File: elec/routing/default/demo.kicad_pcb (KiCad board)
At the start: 4 copper layers, 25 x 25 mm, 34 parts, among them U1 ?, U2 ?, U3 ?, U4 ?, U5 ?, U6 KMR211NGLFS (Tactile Switches), U7 ?, U8 ?

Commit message: [DEMO] tweaks
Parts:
- C1, C15, C19, C2: value 25V 1uF X5R Â±10% 0402 Multilayer Ceramic Capacitors MLCC - SMD/SMT ROHS -> 25V 1uF X5R ±10% 0402 Multilayer Ceramic Capacitors MLCC - SMD/SMT ROHS
- C10, C11, C12, C13, C14, C16, C17, C18, C4, C6, C7: value 16V 100nF X7R Â±10% 0402 Multilayer Ceramic Capacitors MLCC - SMD/SMT ROHS -> 16V 100nF X7R ±10% 0402 Multilayer Ceramic Capacitors MLCC - SMD/SMT ROHS
- C3: value 6.3V 10uF X5R Â±20% 0402 Multilayer Ceramic Capacitors MLCC - SMD/SMT ROHS -> 6.3V 10uF X5R ±20% 0402 Multilayer Ceramic Capacitors MLCC - SMD/SMT ROHS
- C5: value 10V 4.7uF X5R Â±20% 0402 Multilayer Ceramic Capacitors MLCC - SMD/SMT ROHS -> 10V 4.7uF X5R ±20% 0402 Multilayer Ceramic Capacitors MLCC - SMD/SMT ROHS
- C8, C9: value 50V 20pF C0G Â±5% 0402 Multilayer Ceramic Capacitors MLCC - SMD/SMT ROHS -> 50V 20pF C0G ±5% 0402 Multilayer Ceramic Capacitors MLCC - SMD/SMT ROHS
- R1, R2: value 62.5mW Thick Film Resistors 50V Â±100ppm/â Â±1% 5.1kÎ© 0402 Chip Resistor - Surface Mount ROHS -> 62.5mW Thick Film Resistors 50V ±100ppm/℃ ±1% 5.1kΩ 0402 Chip Resistor - Surface Mount ROHS
- R3, R4: value 62.5mW Thick Film Resistors 50V Â±100ppm/â Â±1% 10kÎ© 0402 Chip Resistor - Surface Mount ROHS -> 62.5mW Thick Film Resistors 50V ±100ppm/℃ ±1% 10kΩ 0402 Chip Resistor - Surface Mount ROHS
- R5: value 62.5mW Thick Film Resistors 50V Â±100ppm/â Â±1% 1kÎ© 0402 Chip Resistor - Surface Mount ROHS -> 62.5mW Thick Film Resistors 50V ±100ppm/℃ ±1% 1kΩ 0402 Chip Resistor - Surface Mount ROHS
- R6, R7: value 62.5mW Thick Film Resistors 50V Â±100ppm/â Â±1% 27Î© 0402 Chip Resistor - Surface Mount ROHS -> 62.5mW Thick Film Resistors 50V ±100ppm/℃ ±1% 27Ω 0402 Chip Resistor - Surface Mount ROHS

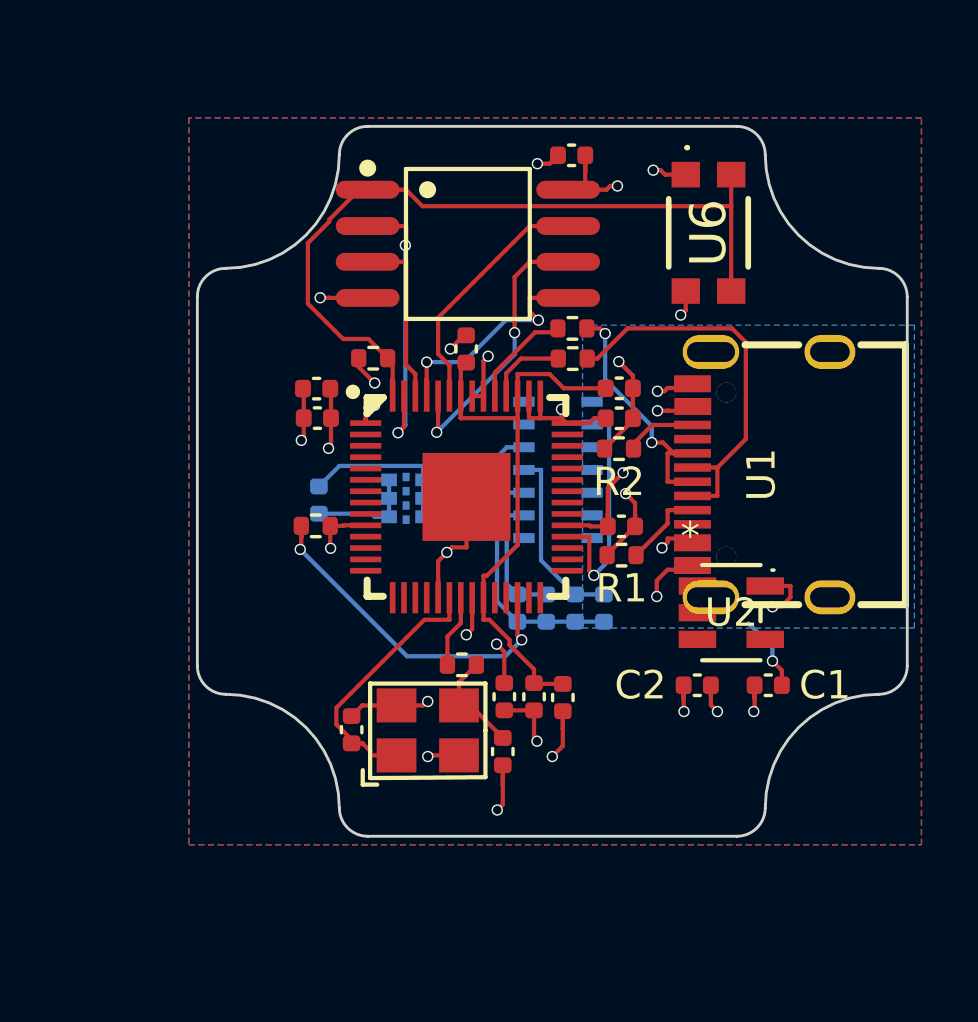
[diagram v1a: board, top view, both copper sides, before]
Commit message: [DEMO] better
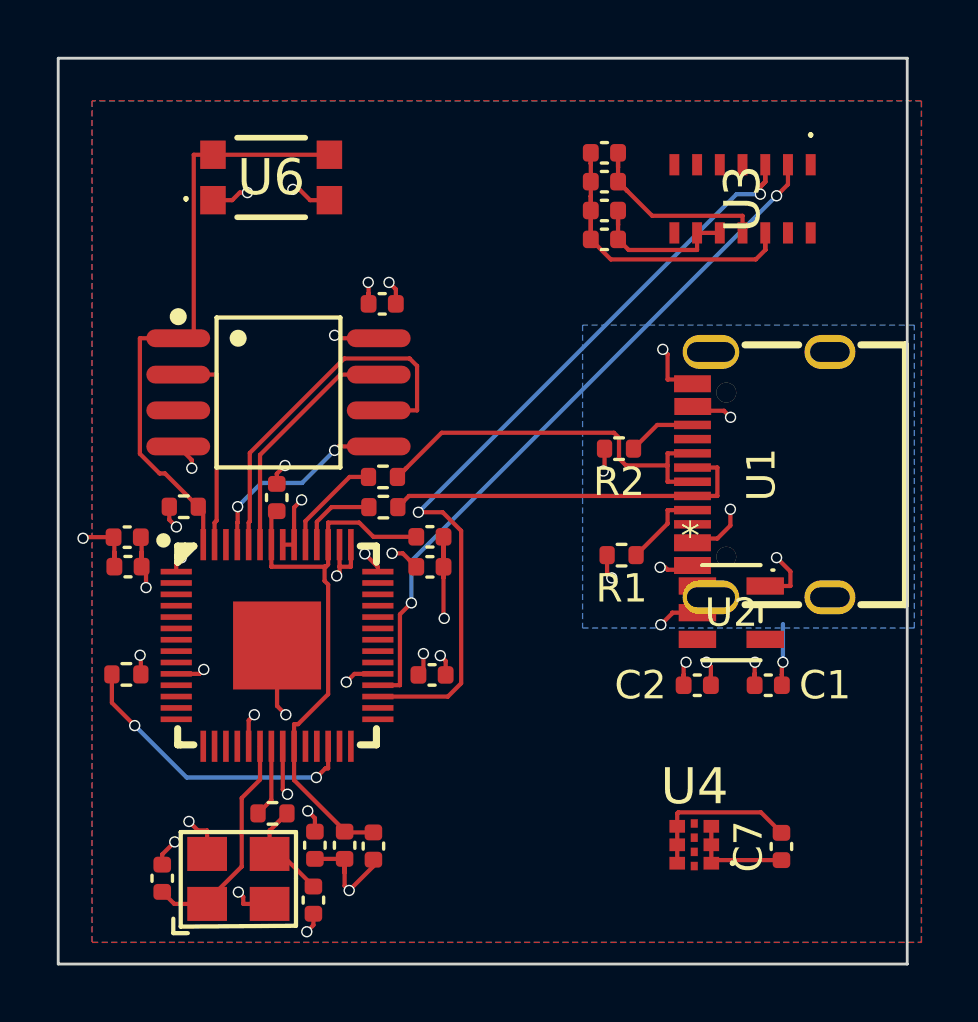
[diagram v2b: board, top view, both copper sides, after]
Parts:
- C3, C4, C5, C6, C7, U3, U4: moved to F.Cu
- moved C7 20.4 mm to (150.6, 115.4)
- moved C3 16.0 mm to (144.3, 90.9), turned to 180 degrees
- moved U4 15.9 mm to (147.5, 115.3), turned to 180 degrees
- moved U6 15.5 mm to (132.6, 91.8), turned to 180 degrees
- moved C4 15.1 mm to (144.3, 91.9), turned to 180 degrees
- moved C5 14.1 mm to (144.3, 93.0), turned to 180 degrees
- moved C6 13.3 mm to (144.3, 94.0), turned to 180 degrees
- moved U3 11.6 mm to (149.2, 92.6), turned to -90 degrees
- moved C13 8.48 mm to (127.6, 105.5)
- moved C8 8.48 mm to (128.8, 116.5)
- moved R4 8.48 mm to (129.5, 103.4)
- moved R7 8.48 mm to (136.6, 103.4)
- moved U5 8.48 mm to (132.8, 108.3)
- moved C10 8.48 mm to (134.1, 115.3)
- moved C12 8.48 mm to (127.5, 104.5)
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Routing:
- net sda: track 0.00 -> 28.9 mm, vias 0 -> 2
- net scl: track 8.34 -> 24.9 mm, vias 1 -> 2
- net io2: track 6.61 -> 0.00 mm
- net microcontroller.rp2040-cs-1: track 27.9 -> 21.8 mm
- net dp: track 8.93 -> 14.3 mm, vias 2 -> 0
- net power_supply-vcc: track 28.2 -> 23.2 mm, vias 12 -> 17
- net io1: track 10.7 -> 7.37 mm, vias 2 -> 0
- net microcontroller.rp2040-sck-1: track 10.6 -> 13.5 mm, vias 2 -> 0
- net sensor.sensor-gnd: track 10.2 -> 13.0 mm
- net run: track 13.1 -> 10.6 mm
- net xin: track 10.2 -> 8.60 mm
- net io0: track 8.60 -> 7.19 mm
- net sensor.sensor-vcc: track 6.50 -> 7.75 mm
- net microcontroller.rp2040.micro-vcc: track 21.7 -> 20.6 mm
- net io3: track 9.39 -> 8.51 mm
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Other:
- board size 25 x 25 mm -> 29.9 x 31.9 mm
